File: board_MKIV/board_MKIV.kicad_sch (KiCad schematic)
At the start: 45 parts, among them J1 1757242, J2 jst-power, J3 JST -SM, J5 1770979, J6 20_pin_90, J7 20-pin-straight, U1 ESP32-DEVKITC-32D, U2 LTV-846S, U3 TLV272CDR, U4 BAT46W, U5 BA&, U6 SH-7070TB

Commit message: update
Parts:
- removed C1, C2: UHE2A470MPD, footprints:PCAP_10x12_5-THRU-ELECT_NCA, symbol custom_library:UHE2A470MPD
- removed C3: 1000pf/3kV, footprints:CAPC3216X180N, symbol CL31B106KAHNNNE:CL31B106KAHNNNE
- removed D1: SS34B-HF, footprints:DO214AASMB_CIP-L, symbol custom_library:SS34B-HF
- removed J7: 20-pin-straight, footprints:20_pin_straight, symbol 20_pin_straight:XC5B-2021
- removed LED1: COM-16347, footprints:COM-16347_SPK, symbol RGB_LED:COM-16347
- removed PS1: REC5A-2405SW_H2, footprints:CONV_REC5A-2405SW_H2, symbol custom_library:REC5A-2405SW_H2
- removed R13, R14, R15, R16: CR1206-FX-1002ELF, footprints:RESC3216X75N, symbol CR1206-FX-1002ELF:CR1206-FX-1002ELF
- removed R7: CRL1206-FW-R330ELF, footprints:RESC3216X70N, symbol CRL1206-FW-R330ELF:CRL1206-FW-R330ELF
- removed RF1, RF2: ~, footprints:PTC_RESET_FUSE, symbol custom_library:reset_fuse
- removed S1: DS01C-254-S-03BE, footprints:SW_DS01C-254-S-03BE, symbol DS01C-254-S-03BE:DS01C-254-S-03BE
- removed S2: PB400EEQR1BLK, footprints:SW_PB400EEQR1BLK, symbol PB400EEQR1BLK:PB400EEQR1BLK
- removed U1: ESP32-DEVKITC-32D, footprints:MODULE_ESP32-DEVKITC-32D, symbol custom_library:ESP32-DEVKITC-32D
- removed U6: SH-7070TB, footprints:SH-7070TB_7P1X7P3_NDC, symbol rot_switch:SH-7070TB
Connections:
- no-connect marks 20 -> 4
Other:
- added sheet ESP-Board (ESP-Board.kicad_sch)
- moved on the sheet: J1, J2, J3, J5, J6, R1, R10, R11, R12, R17, R18, R2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

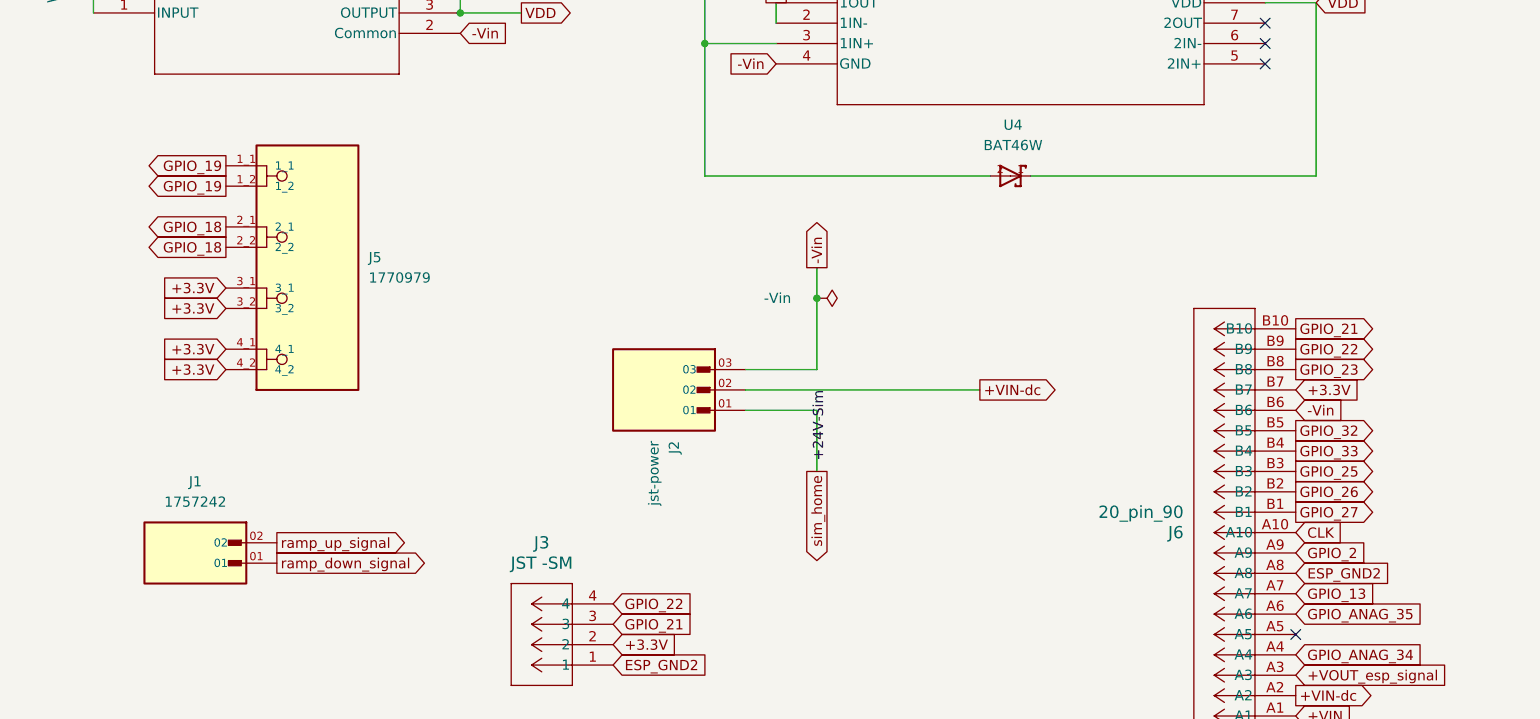
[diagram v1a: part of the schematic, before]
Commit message: MKIV Update
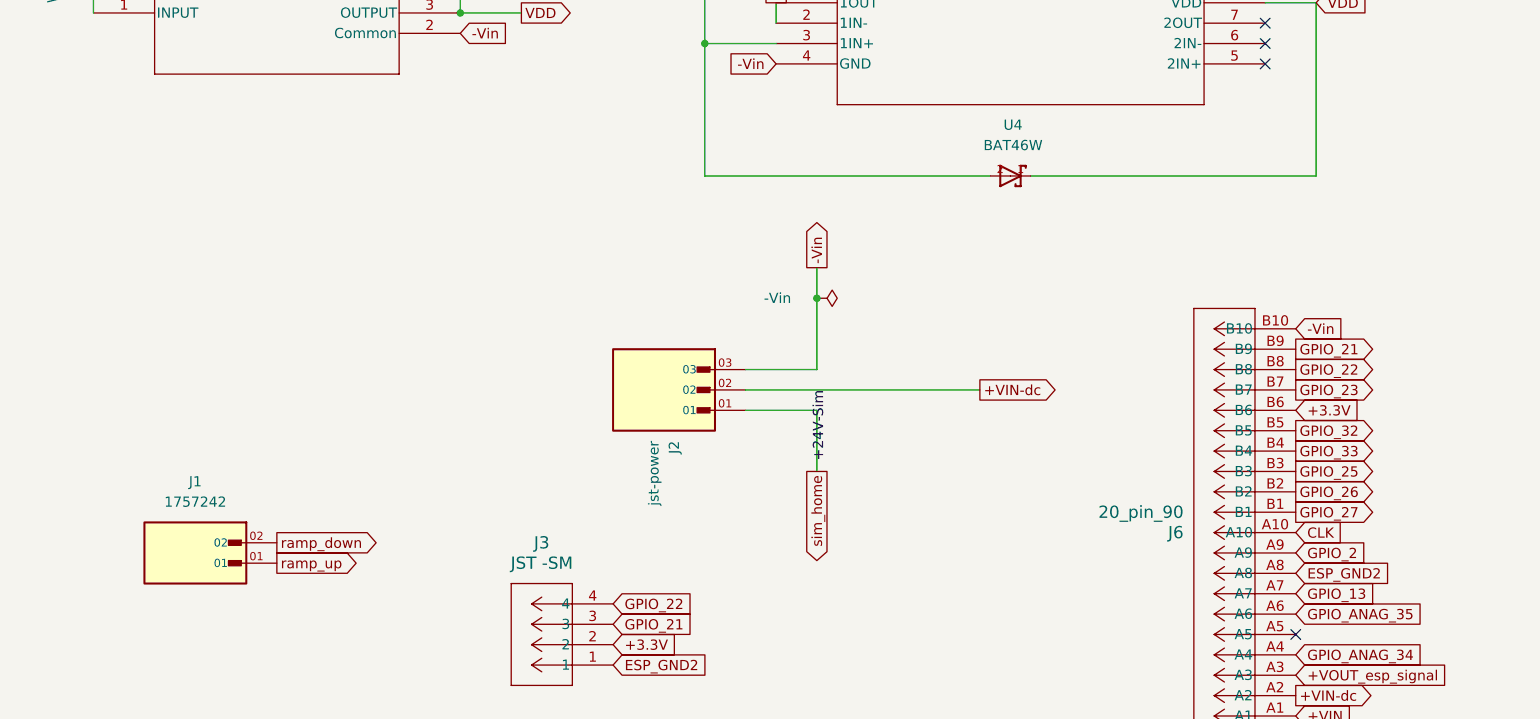
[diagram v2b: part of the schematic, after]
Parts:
- removed J5: 1770979, footprints:PHOENIX_1770979, symbol 1770979:1770979
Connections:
- net ramp_down_signal is gone; now on net ramp_up: J1.01
- net ramp_up_signal is gone; now on net ramp_down: J1.02
- net +3.3V: now also J6.B6; no longer J6.B7
- net -Vin: now also J6.B10; no longer J6.B6
- net GPIO_21: now also J6.B9; no longer J6.B10
- net GPIO_22: now also J6.B8; no longer J6.B9
- net GPIO_23: now also J6.B7; no longer J6.B8
